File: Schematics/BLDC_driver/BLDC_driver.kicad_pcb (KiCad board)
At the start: 2 copper layers, 9 parts, among them J1 DA15_Plug_MountingHoles, J2 Conn_01x02_Pin, Q1 2SC4213, Q2 2SC4213, U1 LM7812_TO220, U2 LM2596S-3.3, U3 CH340C, U4 ESP32-WROOM-32D

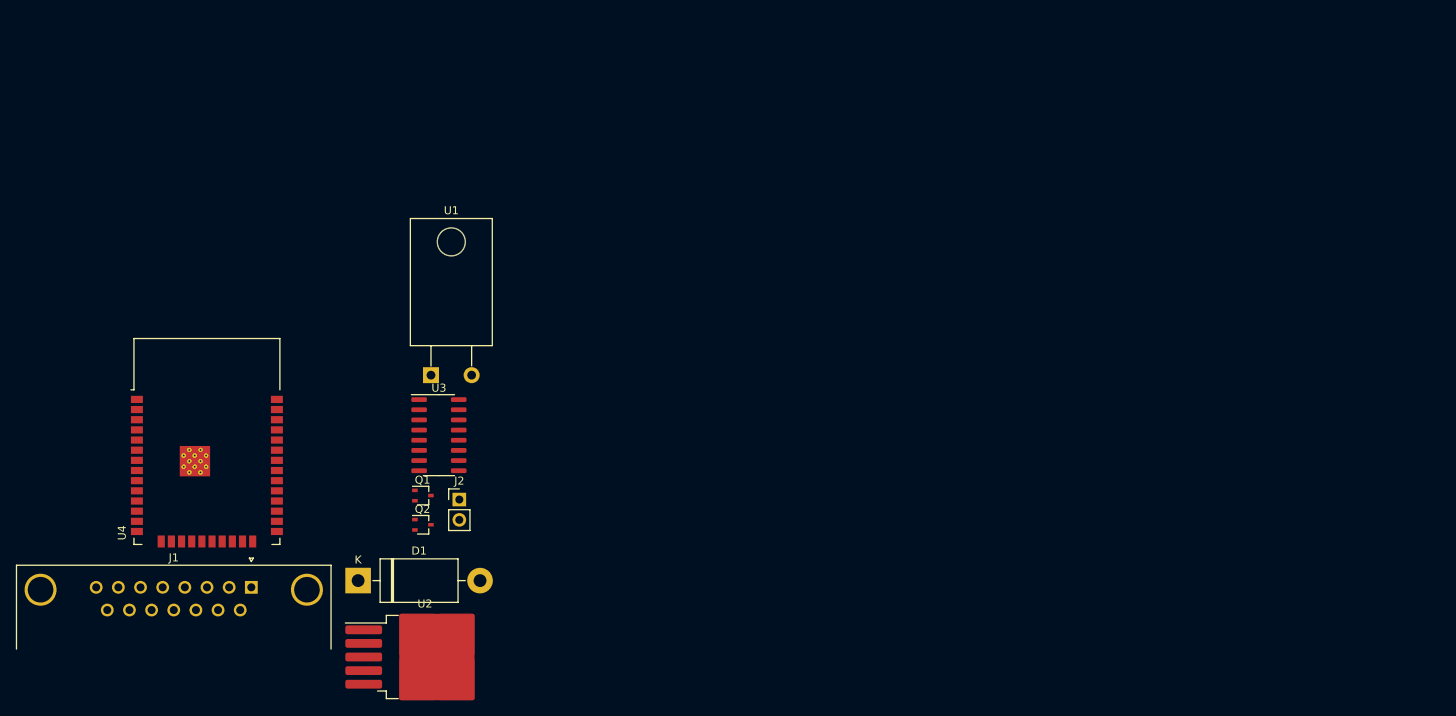
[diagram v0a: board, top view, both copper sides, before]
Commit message: Finished design
Generated gerber files, upgraded to KiCAD 8.0.7 this is final design (hopefully)
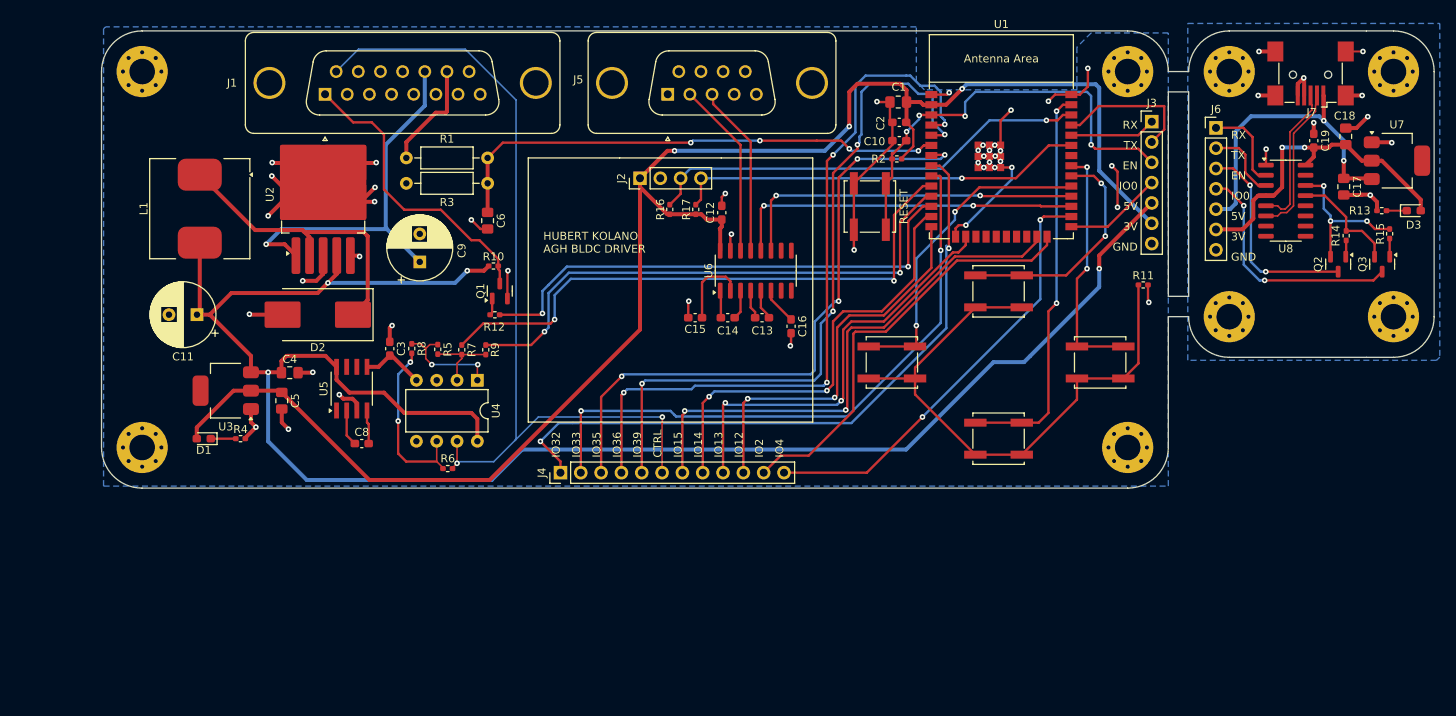
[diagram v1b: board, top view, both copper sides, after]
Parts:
- added C1: 22u, Capacitor_SMD:C_0805_2012Metric_Pad1.18x1.45mm_HandSolder, F.Cu at (145.3, 58.4)
- added C10: 0.1u, Capacitor_SMD:C_0603_1608Metric_Pad1.08x0.95mm_HandSolder, F.Cu at (145.4, 63.2)
- added C11: 220u/35v, Capacitor_THT:CP_Radial_D8.0mm_P3.50mm, F.Cu at (57.7, 85.0)
- added C12: 0.1u, Capacitor_SMD:C_0603_1608Metric_Pad1.08x0.95mm_HandSolder, F.Cu at (123.2, 72.2)
- added C13: 0.1u, Capacitor_SMD:C_0603_1608Metric_Pad1.08x0.95mm_HandSolder, F.Cu at (128.3, 85.4)
- added C14: 0.1u, Capacitor_SMD:C_0603_1608Metric_Pad1.08x0.95mm_HandSolder, F.Cu at (124.0, 85.4)
- added C15: 0.1u, Capacitor_SMD:C_0603_1608Metric_Pad1.08x0.95mm_HandSolder, F.Cu at (119.9, 85.4)
- added C16: 0.1u, Capacitor_SMD:C_0603_1608Metric_Pad1.08x0.95mm_HandSolder, F.Cu at (131.9, 86.5)
- added C17: 22u, Capacitor_SMD:C_0805_2012Metric_Pad1.18x1.45mm_HandSolder, F.Cu at (201.0, 69.0)
- added C18: 22u, Capacitor_SMD:C_0805_2012Metric_Pad1.18x1.45mm_HandSolder, F.Cu at (201.2, 62.7)
- added C19: 0.1u, Capacitor_SMD:C_0603_1608Metric_Pad1.08x0.95mm_HandSolder, F.Cu at (197.2, 63.2)
- added C2: 0.1u, Capacitor_SMD:C_0603_1608Metric_Pad1.08x0.95mm_HandSolder, F.Cu at (145.4, 61.0)
- added C3: 0.1u, Capacitor_SMD:C_0603_1608Metric_Pad1.08x0.95mm_HandSolder, F.Cu at (81.8, 89.2)
- added C4: 22u, Capacitor_SMD:C_0805_2012Metric_Pad1.18x1.45mm_HandSolder, F.Cu at (69.2, 92.2)
- added C5: 22u, Capacitor_SMD:C_0805_2012Metric_Pad1.18x1.45mm_HandSolder, F.Cu at (68.2, 95.8)
- added C6: 22u, Capacitor_SMD:C_0805_2012Metric_Pad1.18x1.45mm_HandSolder, F.Cu at (94.0, 73.2)
- added C8: 0.1u, Capacitor_SMD:C_0603_1608Metric_Pad1.08x0.95mm_HandSolder, F.Cu at (78.2, 101.1)
- added C9: 220u/35v, Capacitor_THT:CP_Radial_D8.0mm_P3.50mm, F.Cu at (85.5, 78.4)
- added D2: B320, Diode_SMD:D_SMC_Handsoldering, F.Cu at (72.8, 85.0)
- added D3: RED, Diode_SMD:D_0603_1608Metric_Pad1.05x0.95mm_HandSolder, F.Cu at (209.8, 72.0)
- added H1: MountingHole, MountingHole:MountingHole_3.2mm_M3_Pad_Via, F.Cu at (50.8, 101.6)
- added H2: MountingHole, MountingHole:MountingHole_3.2mm_M3_Pad_Via, F.Cu at (50.8, 54.6)
- added H3: MountingHole, MountingHole:MountingHole_3.2mm_M3_Pad_Via, F.Cu at (174.0, 54.6)
- added H4: MountingHole, MountingHole:MountingHole_3.2mm_M3_Pad_Via, F.Cu at (174.0, 101.6)
- added H5: MountingHole, MountingHole:MountingHole_3.2mm_M3_Pad_Via, F.Cu at (186.7, 85.2)
- added H6: MountingHole, MountingHole:MountingHole_3.2mm_M3_Pad_Via, F.Cu at (186.7, 54.6)
- added H7: MountingHole, MountingHole:MountingHole_3.2mm_M3_Pad_Via, F.Cu at (207.2, 54.6)
- added H8: MountingHole, MountingHole:MountingHole_3.2mm_M3_Pad_Via, F.Cu at (207.2, 85.2)
- added J3: Programmer IO, Connector_PinHeader_2.54mm:PinHeader_1x07_P2.54mm_Vertical, F.Cu at (177.0, 60.9)
- added J4: unused pins, Connector_PinHeader_2.54mm:PinHeader_1x12_P2.54mm_Vertical, F.Cu at (103.1, 104.8)
- added J5: DE9_Receptacle_MountingHoles, Connector_Dsub:DSUB-9_Female_Vertical_P2.77x2.84mm_MountingHoles, F.Cu at (116.5, 57.5)
- added J6: Conn_01x07_Pin, Connector_PinHeader_2.54mm:PinHeader_1x07_P2.54mm_Vertical, F.Cu at (185.0, 61.6)
- added J7: USB_B_Micro, Connector_USB:USB_Mini-B_Wuerth_65100516121_Horizontal, F.Cu at (196.8, 55.0)
- added L1: 33u, Inductor_SMD:L_Coilcraft_MSS1278T-XXX, F.Cu at (58.0, 71.8)
- added Q3: 2N7002, Package_TO_SOT_SMD:SOT-23, F.Cu at (205.8, 78.7)
- added R1: 10k, Resistor_THT:R_Axial_DIN0207_L6.3mm_D2.5mm_P10.16mm_Horizontal, F.Cu at (83.8, 65.4)
- added R10: 100, Resistor_SMD:R_0402_1005Metric_Pad0.72x0.64mm_HandSolder, F.Cu at (94.7, 78.9)
- added R11: 10k, Resistor_SMD:R_0402_1005Metric_Pad0.72x0.64mm_HandSolder, F.Cu at (175.9, 81.3)
- added R12: 10k, Resistor_SMD:R_0402_1005Metric_Pad0.72x0.64mm_HandSolder, F.Cu at (94.9, 85.0)
- added R13: 10k, Resistor_SMD:R_0402_1005Metric_Pad0.72x0.64mm_HandSolder, F.Cu at (205.8, 72.0)
- added R14: 10k, Resistor_SMD:R_0402_1005Metric_Pad0.72x0.64mm_HandSolder, F.Cu at (201.3, 75.1)
- added R15: 10k, Resistor_SMD:R_0402_1005Metric_Pad0.72x0.64mm_HandSolder, F.Cu at (206.7, 74.9)
- added R16: 3k3, Resistor_SMD:R_0402_1005Metric_Pad0.72x0.64mm_HandSolder, F.Cu at (116.8, 71.8)
- added R17: 3k3, Resistor_SMD:R_0402_1005Metric_Pad0.72x0.64mm_HandSolder, F.Cu at (120.0, 71.8)
- added R2: 10k, Resistor_SMD:R_0402_1005Metric_Pad0.72x0.64mm_HandSolder, F.Cu at (145.1, 65.5)
- added R3: 1k6, Resistor_THT:R_Axial_DIN0207_L6.3mm_D2.5mm_P10.16mm_Horizontal, F.Cu at (94.0, 68.6)
- added R4: 10k, Resistor_SMD:R_0402_1005Metric_Pad0.72x0.64mm_HandSolder, F.Cu at (63.1, 100.5)
- added R5: 7k5, Resistor_SMD:R_0402_1005Metric_Pad0.72x0.64mm_HandSolder, F.Cu at (87.8, 89.3)
- added R6: 10k, Resistor_SMD:R_0402_1005Metric_Pad0.72x0.64mm_HandSolder, F.Cu at (89.0, 104.2)
- added R7: 10k, Resistor_SMD:R_0402_1005Metric_Pad0.72x0.64mm_HandSolder, F.Cu at (90.8, 89.4)
- added R8: 10k, Resistor_SMD:R_0402_1005Metric_Pad0.72x0.64mm_HandSolder, F.Cu at (84.5, 89.2)
- added R9: 10k, Resistor_SMD:R_0402_1005Metric_Pad0.72x0.64mm_HandSolder, F.Cu at (93.8, 89.4)
- added RESET: SW_Push, PCM_Espressif:SW_Push_1P1T_NO_CK_KSC6xxJ22, F.Cu at (141.8, 71.5)
- added SW2: SW_Push, PCM_Espressif:SW_Push_1P1T_NO_CK_KSC6xxJ22, F.Cu at (157.8, 82.1)
- added SW3: SW_Push, PCM_Espressif:SW_Push_1P1T_NO_CK_KSC6xxJ22, F.Cu at (157.8, 100.5)
- added SW4: SW_Push, PCM_Espressif:SW_Push_1P1T_NO_CK_KSC6xxJ22, F.Cu at (170.6, 91.0)
- added SW5: SW_Push, PCM_Espressif:SW_Push_1P1T_NO_CK_KSC6xxJ22, F.Cu at (144.5, 91.0)
- added U5: ICL7660, Package_SO:PowerIntegrations_SO-8, F.Cu at (77.0, 94.2)
- added U6: MAX3232, Package_SO:SOP-16_3.9x9.9mm_P1.27mm, F.Cu at (127.5, 79.5)
- added U7: AMS1117-3.3, Package_TO_SOT_SMD:SOT-223, F.Cu at (207.6, 65.8)
- added U8: CH340C, Package_SO:SOIC-16_3.9x9.9mm_P1.27mm, F.Cu at (193.8, 70.8)
- D1: value 1N5822 -> RED; footprint Diode_THT:D_DO-201AD_P15.24mm_Horizontal -> Diode_SMD:D_0603_1608Metric_Pad1.05x0.95mm_HandSolder
- J1: footprint Connector_Dsub:DSUB-15_Female_Horizontal_P2.77x2.84mm_EdgePinOffset4.94mm_Housed_MountingHolesOffset7.48mm -> Connector_Dsub:DSUB-15_Female_Vertical_P2.77x2.84mm_MountingHoles
- J2: value Conn_01x02_Pin -> Display connectors; footprint Connector_PinHeader_2.54mm:PinHeader_1x02_P2.54mm_Vertical -> Connector_PinHeader_2.54mm:PinHeader_1x04_P2.54mm_Vertical
- Q1, Q2: value 2SC4213 -> 2N7002; footprint Package_TO_SOT_SMD:SOT-323_SC-70 -> Package_TO_SOT_SMD:SOT-23
- U1: value LM7812_TO220 -> ESP32-WROOM-E; footprint Package_TO_SOT_THT:TO-220-2_Horizontal_TabDown -> PCM_Espressif:ESP32-WROOM-32E
- U2: value LM2596S-3.3 -> LM2596S-5
- U3: value CH340C -> AMS1117-3.3; footprint Package_SO:SOIC-16_3.9x9.9mm_P1.27mm -> Package_TO_SOT_SMD:SOT-223
- U4: value ESP32-WROOM-32D -> LM358; footprint RF_Module:ESP32-WROOM-32D -> Package_DIP:DIP-8_W7.62mm
- moved Q2 119.0 mm to (200.3, 78.7), turned to -90 degrees
- moved U1 76.6 mm to (158.2, 64.5)
- moved J1 62.3 mm to (73.7, 57.5), turned to 180 degrees
- moved U2 59.2 mm to (73.4, 70.0), turned to 90 degrees
- moved J2 46.1 mm to (113.0, 67.9), turned to 90 degrees
- moved U4 35.4 mm to (92.7, 93.2), turned to -90 degrees
- moved Q1 27.3 mm to (95.5, 82.0), turned to 90 degrees
- moved U3 27.2 mm to (61.2, 94.5), turned to 180 degrees
- moved D1 26.2 mm to (58.5, 100.5), turned to 180 degrees
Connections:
- D1 pad 2: GND -> +3.3V
- J2 pad 1: GND -> +3.3V
- J2 pad 2: +24V -> GND
- Q1 pad 2: /DTR -> GND
- Q1 pad 3: unconnected-(Q1-C-Pad3) -> /DIR
- Q2 pad 3: unconnected-(Q2-C-Pad3) -> /EN USB
- U1 pad 1: unconnected-(U1-VI-Pad1) -> GND
- U1 pad 2: unconnected-(U1-GND-Pad2) -> +3.3V
- U2 pad 1: Net-(J3-Pin_2) -> +24V
- U2 pad 2: Net-(D1-K) -> Net-(D2-K)
- U2 pad 4: +3V3 -> +5V
- U3 pad 2: Net-(U3-TXD) -> +3.3V
- U3 pad 3: Net-(U3-RXD) -> +5V
- U3 pad 4: +3V3 -> (no net)
- U4 pad 1: Net-(U4-GND-Pad1) -> Net-(R5-Pad2)
- U4 pad 3: unconnected-(U4-EN-Pad3) -> GND
- U4 pad 4: unconnected-(U4-SENSOR_VP-Pad4) -> -5V
- U4 pad 5: unconnected-(U4-SENSOR_VN-Pad5) -> GND
- U4 pad 6: unconnected-(U4-IO34-Pad6) -> Net-(U4B--)
- U4 pad 7: unconnected-(U4-IO35-Pad7) -> /CTRL
- U4 pad 8: unconnected-(U4-IO32-Pad8) -> +5V
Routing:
- net +5V: track 0.00 -> 236.5 mm, vias 0 -> 4
- net +3.3V: track 0.00 -> 202.8 mm, vias 0 -> 3
- net GND: track 0.00 -> 131.6 mm, vias 0 -> 43
- net /CTRL: track 0.00 -> 107.6 mm, vias 0 -> 2
- net /IO36: track 0.00 -> 92.6 mm, vias 0 -> 4
- net /IO39: track 0.00 -> 88.6 mm, vias 0 -> 4
- net /IO32: track 0.00 -> 84.1 mm, vias 0 -> 2
- net /IO35: track 0.00 -> 79.3 mm, vias 0 -> 4
- net /IO33: track 0.00 -> 77.3 mm, vias 0 -> 2
- net /DAC1: track 0.00 -> 73.7 mm, vias 0 -> 2
- net Net-(R11-Pad1): track 0.00 -> 72.7 mm
- net /DAC2: track 0.00 -> 69.6 mm, vias 0 -> 2
- net /IO15: track 0.00 -> 67.2 mm, vias 0 -> 2
- net /DIR control: track 0.00 -> 64.5 mm, vias 0 -> 2
- net /RPM DIVIDED: track 0.00 -> 64.0 mm, vias 0 -> 4
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- added copper zone on B.Cu, net GND
- added copper zone on B.Cu, net GND1
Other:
- board outline added: 166.6 x 57.2 mm
- board text added: "3V"
- board text added: "5V"
- board text added: "CTRL"
- board text added: "EN"
- board text added: "GND"
- board text added: "HUBERT KOLANO AGH BLDC DRIVER"
- board text added: "IO0"
- board text added: "IO12"
- board text added: "IO13"
- board text added: "IO14"
- board text added: "IO15"
- board text added: "IO2"
- board text added: "IO32"
- board text added: "IO33"
- board text added: "IO35"
- board text added: "IO36"
- board text added: "IO39"
- board text added: "IO4"
- board text added: "RX"
- board text added: "TX"
